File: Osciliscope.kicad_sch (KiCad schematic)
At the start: 32 parts, among them J1 U.FL, J2 Conn_01x04_Socket, J3 U.FL, J4 Conn_01x04_Socket, SW1 SW_Rotary_1x8_MP, SW2 SW_Rotary_1x8_MP, SW3 SW_Nidec_CAS-120A1, SW4 SW_Nidec_CAS-120A1, U1 MCP1700x-330xxMB, U2 ADC082S101, U5 TLV9061xDBV, U7 TLV9061xDBV, U8 MCP4251-104E/ML-ND

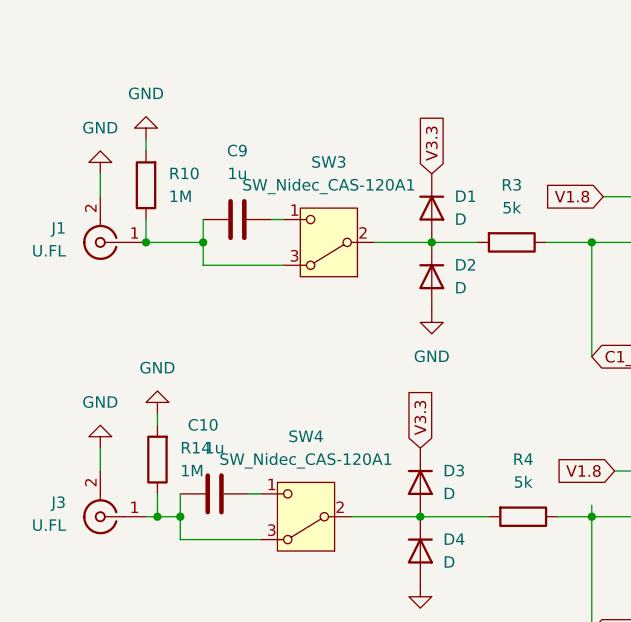
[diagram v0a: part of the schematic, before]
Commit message: more small changes
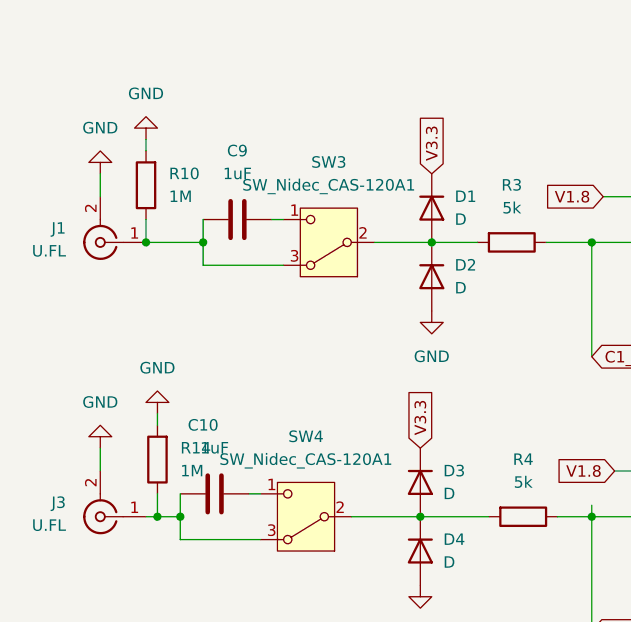
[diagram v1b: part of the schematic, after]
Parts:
- C10, C9: value 1u -> 1uF
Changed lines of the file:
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@@
 			)
 		)
-		(property "Datasheet" "https://eecs.engineering.oregonstate.edu/education/inventory_datasheets/P1502744917.pdf"
+		(property "Datasheet" "https://mm.digikey.com/Volume0/opasdata/d220001/medias/docus/609/CL05A105KO5NNNC_Spec_5-2-19.pdf"
 			(at 143.51 92.71 0)
 			(effects
@@
 			)
 		)
-		(property "Datasheet" "https://eecs.engineering.oregonstate.edu/education/inventory_datasheets/P1502744917.pdf"
+		(property "Datasheet" "https://mm.digikey.com/Volume0/opasdata/d220001/medias/docus/609/CL05A105KO5NNNC_Spec_5-2-19.pdf"
 			(at 149.86 48.26 0)
 			(effects
@@
 			)
 		)
-		(property "Datasheet" "https://eecs.engineering.oregonstate.edu/education/inventory_datasheets/P1502744917.pdf"
+		(property "Datasheet" "https://mm.digikey.com/Volume0/opasdata/d220001/medias/docus/609/CL05A105KO5NNNC_Spec_5-2-19.pdf"
 			(at 129.54 54.61 0)
 			(effects
@@
 			)
 		)
-		(property "Datasheet" "https://eecs.engineering.oregonstate.edu/education/inventory_datasheets/P1502744917.pdf"
+		(property "Datasheet" "https://mm.digikey.com/Volume0/opasdata/d220001/medias/docus/609/CL05A105KO5NNNC_Spec_5-2-19.pdf"
 			(at 129.54 62.23 0)
 			(effects
@@
 			)
 		)
-		(property "Datasheet" "https://eecs.engineering.oregonstate.edu/education/inventory_datasheets/P1502744917.pdf"
+		(property "Datasheet" "https://mm.digikey.com/Volume0/opasdata/d220001/medias/docus/609/CL05A105KO5NNNC_Spec_5-2-19.pdf"
 			(at 212.09 48.26 0)
 			(effects
@@
 			)
 		)
-		(property "Value" "1u"
+		(property "Value" "1uF"
 			(at 38.1 53.34 90)
 			(effects
@@
 			)
 		)
-		(property "Datasheet" "~"
+		(property "Datasheet" "https://mm.digikey.com/Volume0/opasdata/d220001/medias/docus/609/CL05A105KO5NNNC_Spec_5-2-19.pdf"
 			(at 38.1 58.42 0)
 			(effects
@@
 			)
 		)
-		(property "Datasheet" "~"
+		(property "Datasheet" "https://yageogroup.com/content/datasheet/asset/file/PYU-RT_1-TO-0-01_ROHS_L"
 			(at 68.58 60.96 0)
 			(effects
@@
 			)
 		)
-		(property "Datasheet" "~"
+		(property "Datasheet" "https://industrial.panasonic.com/cdbs/www-data/pdf/RDM0000/AOA0000C307.pdf"
 			(at 27.94 54.61 0)
 			(effects
@@
 			)
 		)
-		(property "Datasheet" "~"
+		(property "Datasheet" "https://www.vishay.com/docs/20035/dcrcwe3.pdf"
 			(at 119.38 54.61 0)
 			(effects
@@
 			)
 		)
-		(property "Datasheet" "~"
+		(property "Datasheet" "https://yageogroup.com/content/datasheet/asset/file/PYU-RT_1-TO-0-01_ROHS_L"
 			(at 69.85 91.44 0)
 			(effects
@@
 			)
 		)
-		(property "Datasheet" "~"
+		(property "Datasheet" "https://industrial.panasonic.com/cdbs/www-data/pdf/RDM0000/AOA0000C307.pdf"
 			(at 29.21 85.09 0)
 			(effects
@@
 			)
 		)
-		(property "Datasheet" "https://eecs.engineering.oregonstate.edu/education/inventory_datasheets/P1502744917.pdf"
+		(property "Datasheet" "https://mm.digikey.com/Volume0/opasdata/d220001/medias/docus/609/CL05A105KO5NNNC_Spec_5-2-19.pdf"
 			(at 201.93 48.26 0)
 			(effects
@@
 			)
 		)
-		(property "Datasheet" "https://eecs.engineering.oregonstate.edu/education/inventory_datasheets/P1502744917.pdf"
+		(property "Datasheet" "https://mm.digikey.com/Volume0/opasdata/d220001/medias/docus/609/CL05A105KO5NNNC_Spec_5-2-19.pdf"
 			(at 190.5 48.26 0)
 			(effects
@@
 			)
 		)
-		(property "Datasheet" "~"
+		(property "Datasheet" "https://www.vishay.com/docs/20035/dcrcwe3.pdf"
 			(at 119.38 62.23 0)
 			(effects
@@
 			)
 		)
-		(property "Value" "1u"
+		(property "Value" "1uF"
 			(at 35.56 83.82 90)
 			(effects
@@
 			)
 		)
-		(property "Datasheet" "~"
+		(property "Datasheet" "https://mm.digikey.com/Volume0/opasdata/d220001/medias/docus/609/CL05A105KO5NNNC_Spec_5-2-19.pdf"
 			(at 35.56 88.9 0)
 			(effects
